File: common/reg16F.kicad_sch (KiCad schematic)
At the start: 8 parts, among them U17 74AHC1G08, U18 SN74AHC16374DGGR

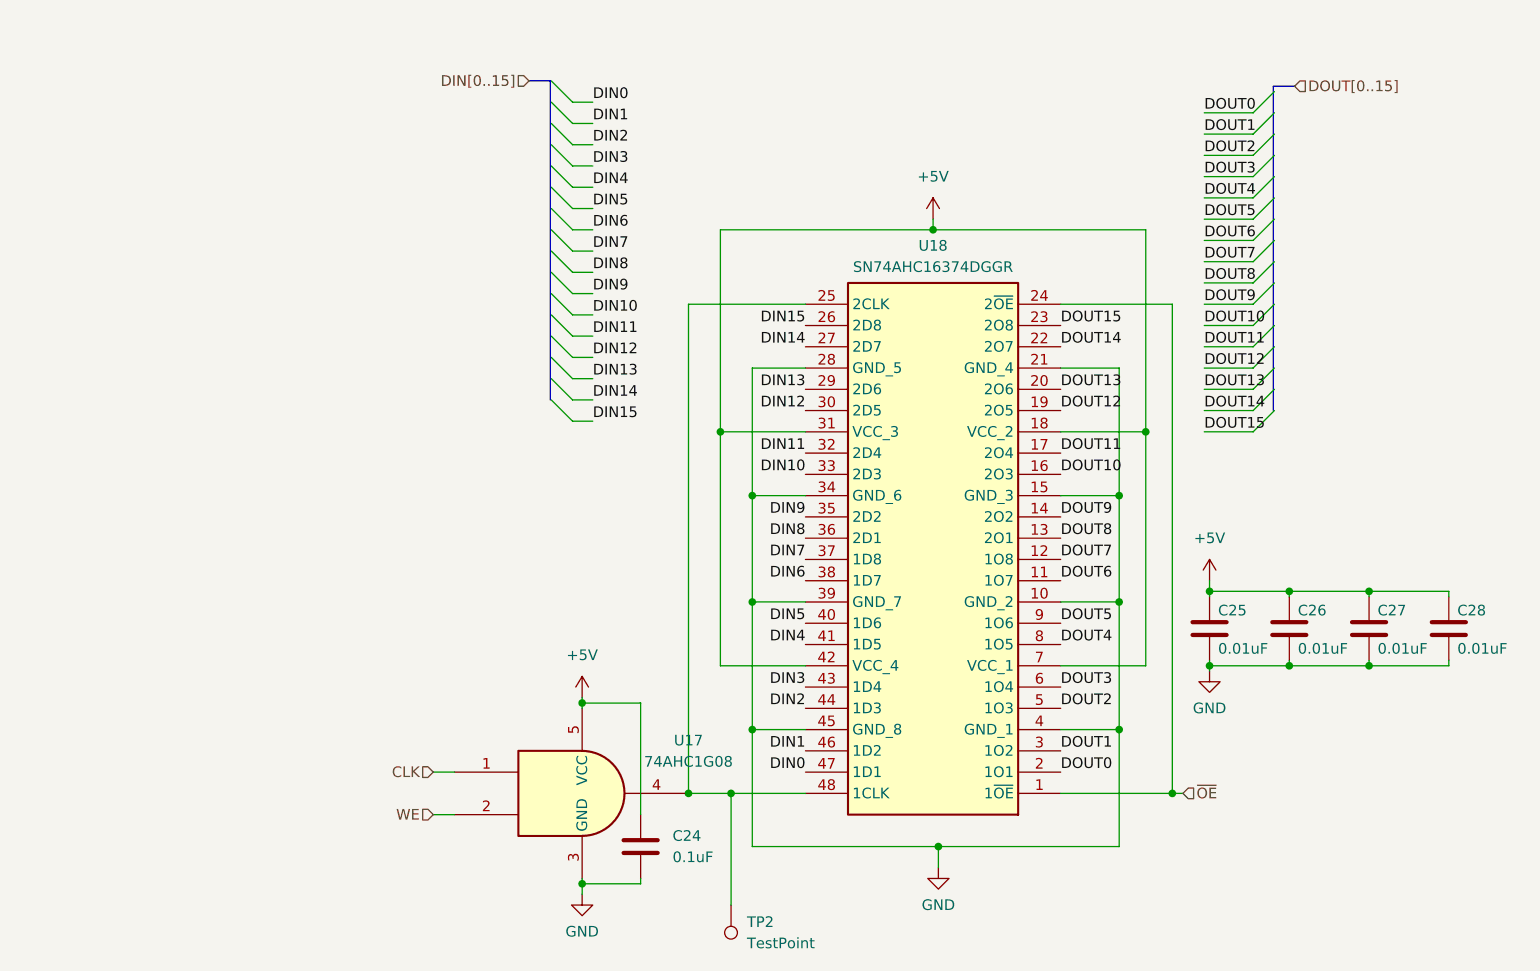
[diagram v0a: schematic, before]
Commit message: Made tri-state and register schematic look nice
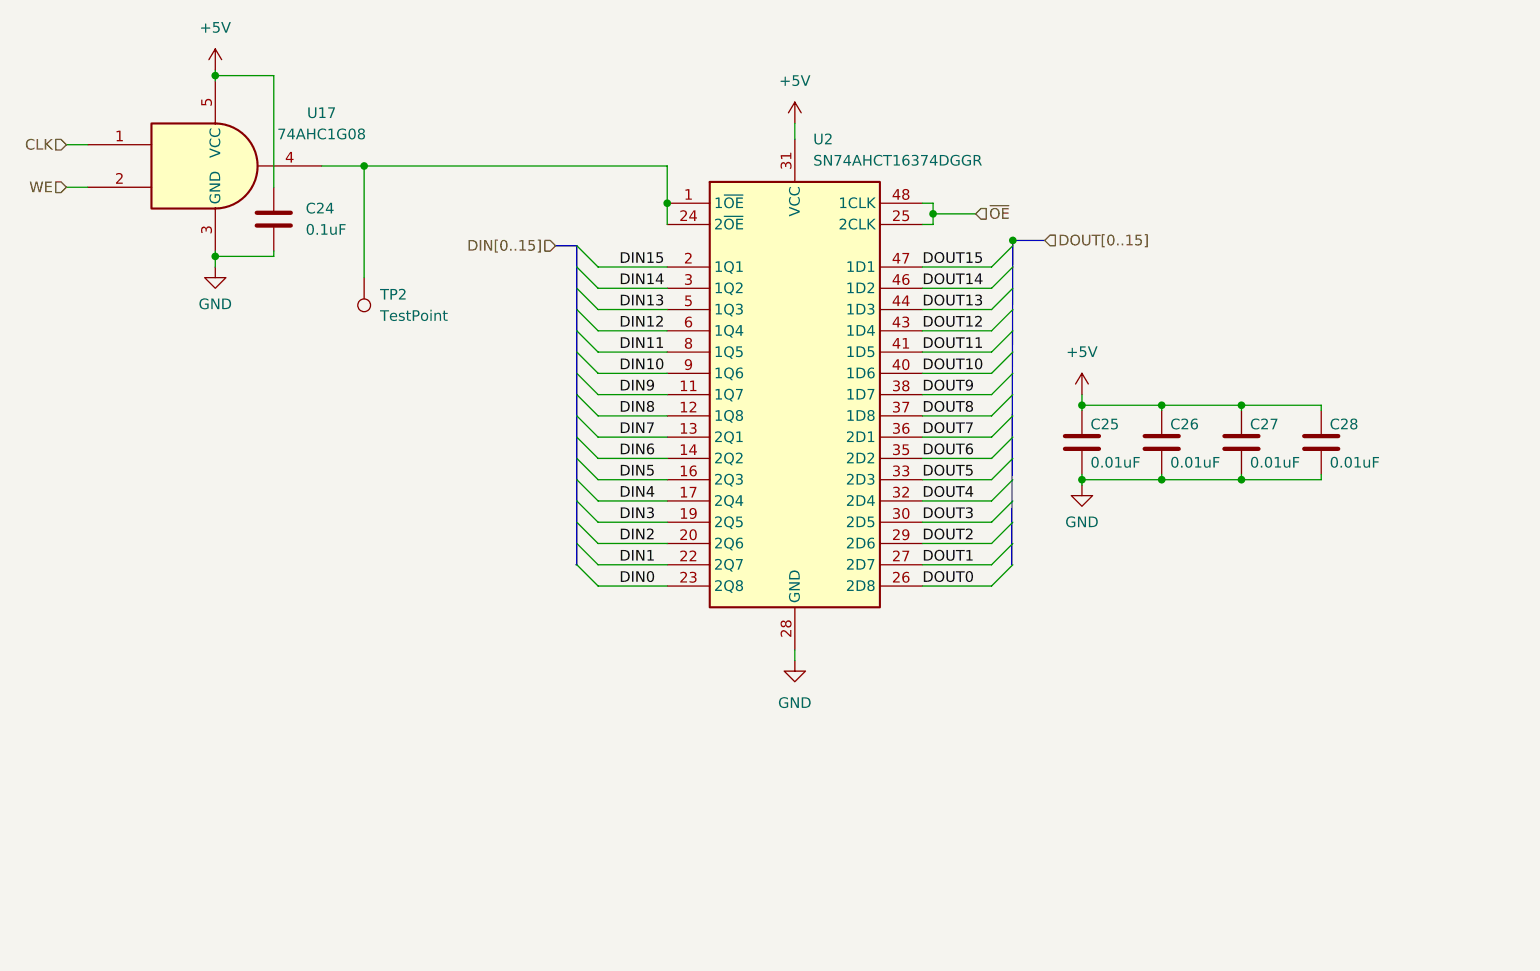
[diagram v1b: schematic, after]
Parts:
- removed U18: SN74AHC16374DGGR, Package_SO:TSSOP-48_6.1x12.5mm_P0.5mm, symbol 74FCT16374CTPVG:74FCT16374CTPVG
- added U2: SN74AHCT16374DGGR, Package_SO:TSSOP-48_6.1x12.5mm_P0.5mm, symbol 74FCT16374CTPVG:74FCT16374CTPVG
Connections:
- net +5V: now also U2.18 (VCC_2), U2.31 (VCC), U2.42 (VCC_4), U2.7 (VCC_1)
- net DIN0: now also U2.23 (2Q8)
- net DIN1: now also U2.22 (2Q7)
- net DIN10: now also U2.9 (1Q6)
- net DIN11: now also U2.8 (1Q5)
- net DIN12: now also U2.6 (1Q4)
- net DIN13: now also U2.5 (1Q3)
- net DIN14: now also U2.3 (1Q2)
- net DIN15: now also U2.2 (1Q1)
- net DIN2: now also U2.20 (2Q6)
- net DIN3: now also U2.19 (2Q5)
- net DIN4: now also U2.17 (2Q4)
- net DIN5: now also U2.16 (2Q3)
- net DIN6: now also U2.14 (2Q2)
- net DIN7: now also U2.13 (2Q1)
- net DIN8: now also U2.12 (1Q8)
- net DIN9: now also U2.11 (1Q7)
- net DOUT0: now also U2.26 (2D8)
- net DOUT1: now also U2.27 (2D7)
- net DOUT10: now also U2.40 (1D6)
- net DOUT11: now also U2.41 (1D5)
- net DOUT12: now also U2.43 (1D4)
- net DOUT13: now also U2.44 (1D3)
- net DOUT14: now also U2.46 (1D2)
- net DOUT15: now also U2.47 (1D1)
- net DOUT2: now also U2.29 (2D6)
- net DOUT3: now also U2.30 (2D5)
- net DOUT4: now also U2.32 (2D4)
- net DOUT5: now also U2.33 (2D3)
- net DOUT6: now also U2.35 (2D2)
- net DOUT7: now also U2.36 (2D1)
- net DOUT8: now also U2.37 (1D8)
- net DOUT9: now also U2.38 (1D7)
- net GND: now also U2.10 (GND_2), U2.15 (GND_3), U2.21 (GND_4), U2.28 (GND), U2.34 (GND_6), U2.39 (GND_7), U2.4 (GND_1), U2.45 (GND_8)
- net ~{OE}: now also U2.25 (2CLK), U2.48 (1CLK)
- net at TP2.1, U17.4: now also U2.1 (1~{OE}), U2.24 (2~{OE})
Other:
- moved on the sheet: C24, C25, C26, C27, C28, TP2, U17
